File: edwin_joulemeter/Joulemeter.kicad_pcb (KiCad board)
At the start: 2 copper layers, 159.8 x 99.8 mm, 54 parts, among them J1 XT60-M, J2 22035035, J3 22035035, J4 XT60-M, U1 INA240A1PWR, U2 REF2033QDDCRQ1, U3 MCP6286T-E/OT, U4 PADS131M04QPWRQ1

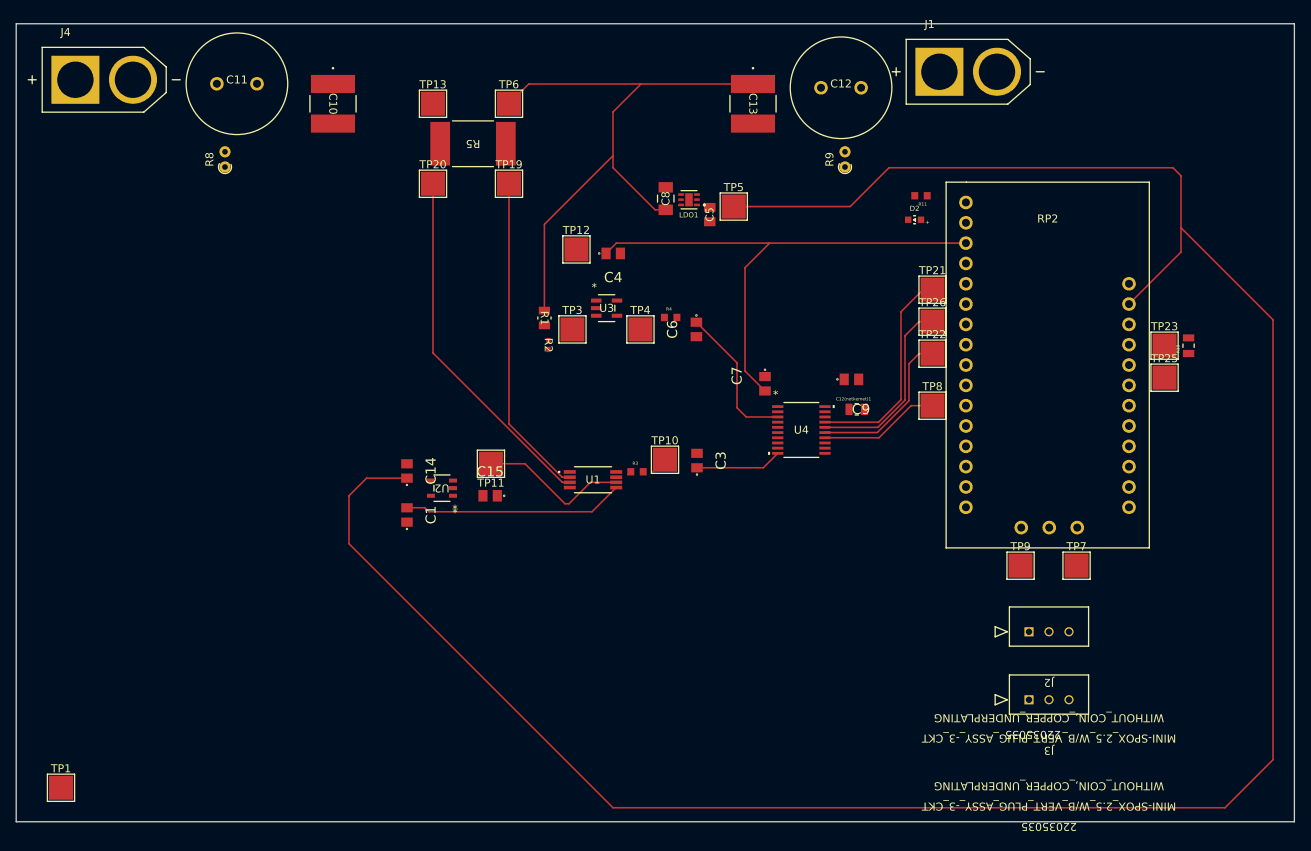
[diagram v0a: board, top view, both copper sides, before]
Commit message: pcb 1/20/25
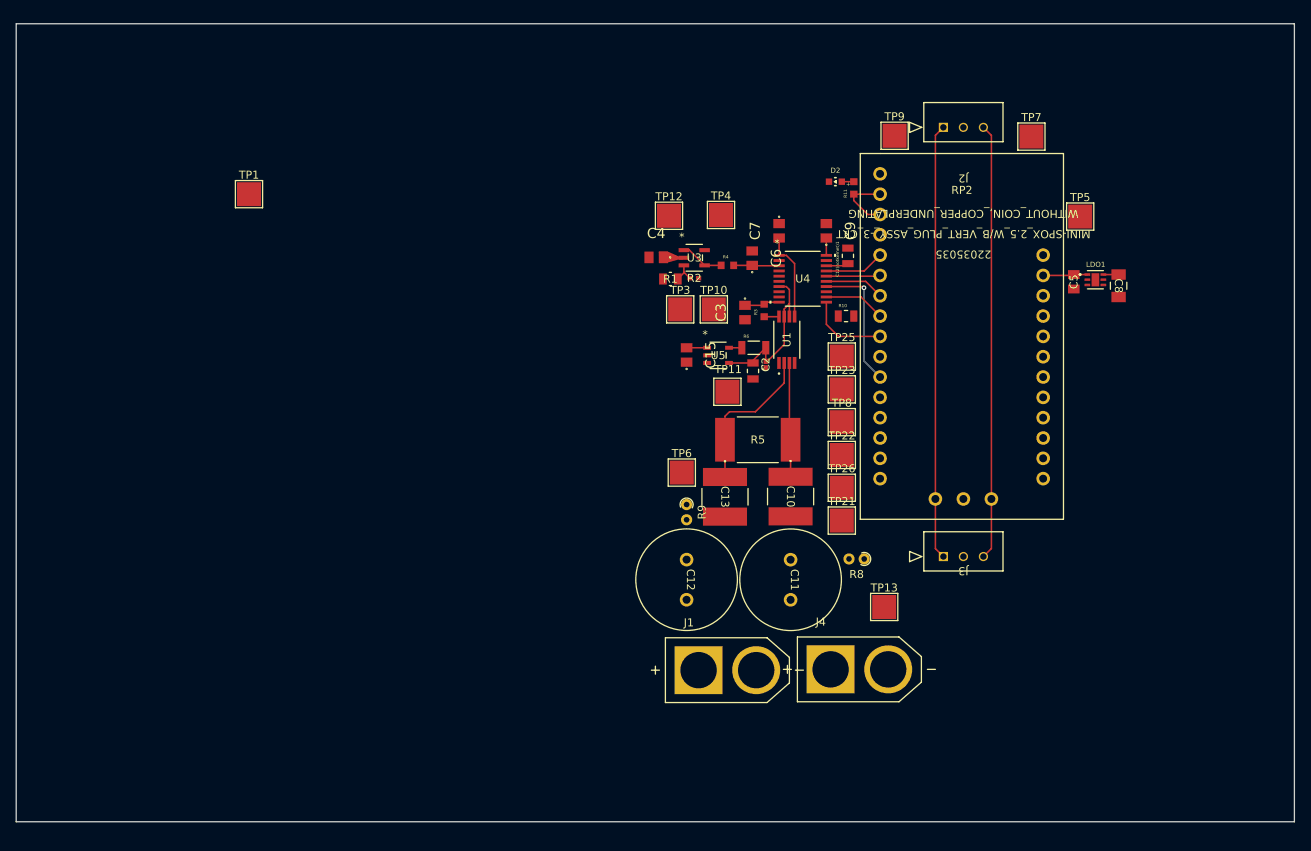
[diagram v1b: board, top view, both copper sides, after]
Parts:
- removed C1, C14: 0.1uF,50V, SMV_Passives:Cap0805
- removed TP19, TP20: TestPoint, TestPoint:TestPoint_Pad_3.0x3.0mm
- removed U2: REF2033QDDCRQ1, SMV_ICs:SOT-23-THIN-5_DDC_TEX
- added C2: 0.47uF, 6.3V, SMV_Passives:CAPC10555_55N_KEM, F.Cu at (115.1, 74.1)
- added R6: 1Mohm, 0.25W, SMV_Passives:RESC3015X65N, F.Cu at (113.6, 72.0)
- added R7: 370kohm, 0.125W, SMV_Passives:RESC2012X50N, F.Cu at (113.5, 74.9)
- added U5: TLV709A01DBVR, SMV_ICs:SOT-23-5_DBV_TEX, F.Cu at (109.1, 72.9)
- moved J4 119.8 mm to (126.8, 112.2)
- moved R8 93.7 mm to (127.4, 98.4), turned to 180 degrees
- moved C11 92.9 mm to (118.2, 101.0), turned to -90 degrees
- moved TP13 84.5 mm to (129.9, 104.4)
- moved J1 80.6 mm to (110.3, 112.3)
- moved TP1 77.8 mm to (50.5, 52.8)
- moved C10 75.4 mm to (118.2, 90.6)
- moved C12 64.5 mm to (105.2, 101.0), turned to -90 degrees
- moved J2 64.0 mm to (137.3, 44.4)
- moved C8 57.6 mm to (159.2, 64.2), turned to -90 degrees
- moved TP9 56.0 mm to (131.2, 45.5)
- moved TP7 53.9 mm to (148.3, 45.6)
- moved LDO1 51.8 mm to (156.3, 63.5), turned to 0 degrees
- moved R5 51.3 mm to (114.1, 83.5), turned to 0 degrees
- moved TP6 50.9 mm to (104.6, 87.6)
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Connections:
- C15 pad 2: +1V65 -> +3V3
- RP2 pad 20: unconnected-(RP2-D24-Pad20) -> /GPIO_RESET
- RP2 pad 21: unconnected-(RP2-A3-Pad21) -> /CS
- RP2 pad 4: /CS -> unconnected-(RP2-D13-Pad4)
- RP2 pad 5: /GPIO_RESET -> unconnected-(RP2-D12-Pad5)
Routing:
- net +5V: track 294.1 -> 5.58 mm
- net +48V: track 115.5 -> 21.1 mm
- net +3V3: track 94.6 -> 24.1 mm
- net /CAN_L: track 0.00 -> 54.5 mm
- net /CAN_H: track 0.00 -> 54.5 mm
- net /SHUNT_OUT: track 45.0 -> 14.3 mm
- net /GPIO_CLKIN: track 26.7 -> 7.54 mm
- net /MOSI: track 24.1 -> 6.75 mm
- net /MISO: track 20.2 -> 7.46 mm
- net /V_ADC: track 18.4 -> 5.70 mm
- net /GPIO_RESET: track 0.00 -> 10.1 mm
- net /I_ADC: track 13.0 -> 4.43 mm
- net /CS: track 0.00 -> 7.71 mm
- net /OP_AMP: track 0.00 -> 5.45 mm
- net Net-(U3-VIN+): track 0.00 -> 3.07 mm
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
